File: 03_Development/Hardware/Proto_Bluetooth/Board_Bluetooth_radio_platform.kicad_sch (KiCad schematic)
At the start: 51 parts, among them J1 Conn_01x02, J10 Conn_01x03, J11 HMI_rotaryEncoder_1, J12 HMI_rotaryEncoder_1, J13 Conn_01x08_epaper, J17 Conn_01x02, J19 Conn_01x02_rn52_usb, J2 Conn_01x08, J3 BT_RN52_connector_left, J4 Conn_01x02, J5 BT_RN52_connector_right, J6 FM_interface, J7 BT_debug_connector, J8 BT_extension_connector, J9 SYS_debug_connector, SW1 SW_Push, U1 LM317_TO-220, U2 NXE2S1205MC

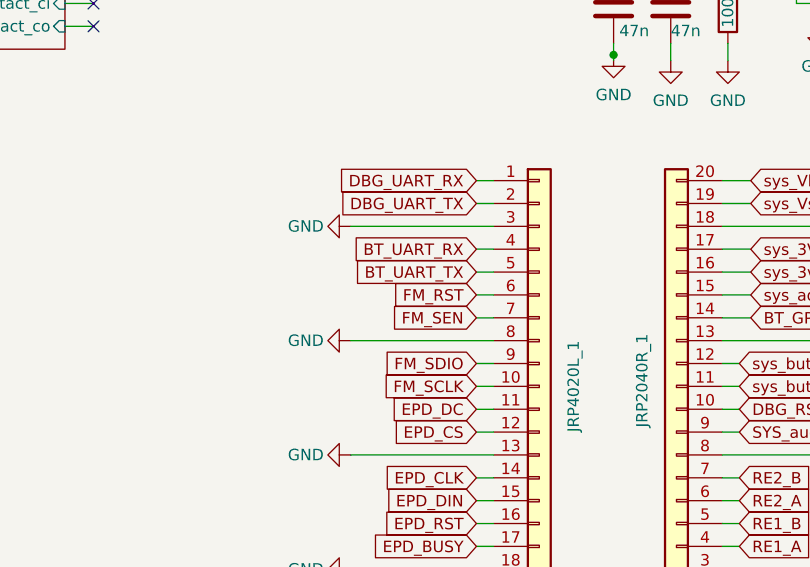
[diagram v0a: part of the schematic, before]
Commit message: [HDW_38] Fix Bt communication wires
Bluetooth Rx pin connected to GPIO4 of RP240
Bluetooth Tx pin connected to GPIO5 of RP2040
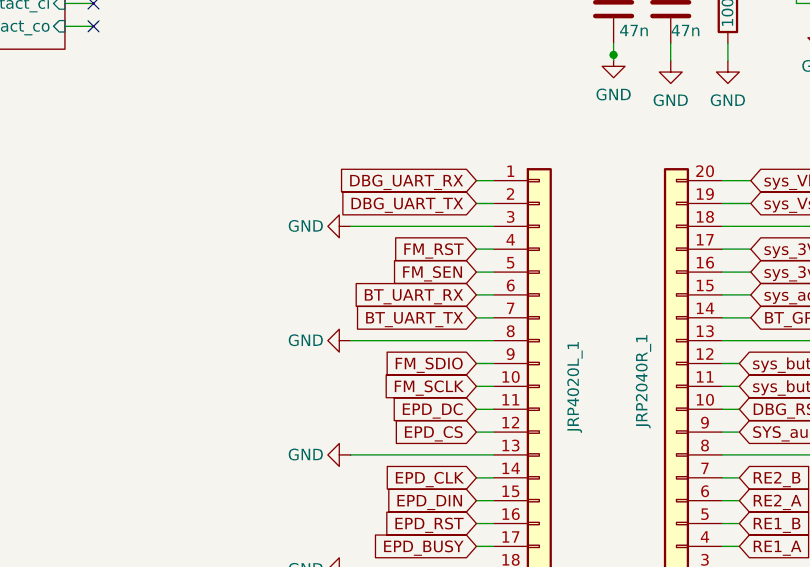
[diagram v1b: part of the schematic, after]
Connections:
- net BT_UART_RX: now also JRP4020L_1.6 (Pin_6); no longer JRP4020L_1.4 (Pin_4)
- net BT_UART_TX: now also JRP4020L_1.7 (Pin_7); no longer JRP4020L_1.5 (Pin_5)
- net FM_RST: now also JRP4020L_1.4 (Pin_4); no longer JRP4020L_1.6 (Pin_6)
- net FM_SEN: now also JRP4020L_1.5 (Pin_5); no longer JRP4020L_1.7 (Pin_7)
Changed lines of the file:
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@@
+    )
+  )
+  (global_label "BT_UART_RX" (shape input) (at 223.52 113.03 180) (fields_autoplaced)
+    (effects (font (size 1.27 1.27)) (justify right))
+    (property "Intersheet References" "${INTERSHEET_REFS}" (id 0) (at 209.7979 112.9506 0)
+      (effects (font (size 1.27 1.27)) (justify right) hide)
     )
   )
@@
     )
   )
-  (global_label "BT_UART_RX" (shape input) (at 223.52 107.95 180) (fields_autoplaced)
-    (effects (font (size 1.27 1.27)) (justify right))
-    (property "Intersheet References" "${INTERSHEET_REFS}" (id 0) (at 209.7979 107.8706 0)
+  (global_label "FM_SEN" (shape input) (at 223.52 110.49 180) (fields_autoplaced)
+    (effects (font (size 1.27 1.27)) (justify right))
+    (property "Intersheet References" "${INTERSHEET_REFS}" (id 0) (at 213.9102 110.4106 0)
+      (effects (font (size 1.27 1.27)) (justify right) hide)
+    )
+  )
+  (global_label "FM_RST" (shape input) (at 223.52 107.95 180) (fields_autoplaced)
+    (effects (font (size 1.27 1.27)) (justify right))
+    (property "Intersheet References" "${INTERSHEET_REFS}" (id 0) (at 214.1521 107.8706 0)
       (effects (font (size 1.27 1.27)) (justify right) hide)
     )
@@
     )
   )
-  (global_label "FM_RST" (shape input) (at 223.52 113.03 180) (fields_autoplaced)
-    (effects (font (size 1.27 1.27)) (justify right))
-    (property "Intersheet References" "${INTERSHEET_REFS}" (id 0) (at 214.1521 112.9506 0)
-      (effects (font (size 1.27 1.27)) (justify right) hide)
-    )
-  )
   (global_label "BT_PWREN" (shape input) (at 40.005 188.595 180) (fields_autoplaced)
     (effects (font (size 1.27 1.27)) (justify right))
@@
     )
   )
-  (global_label "FM_SEN" (shape input) (at 223.52 115.57 180) (fields_autoplaced)
-    (effects (font (size 1.27 1.27)) (justify right))
-    (property "Intersheet References" "${INTERSHEET_REFS}" (id 0) (at 213.9102 115.4906 0)
-      (effects (font (size 1.27 1.27)) (justify right) hide)
-    )
-  )
   (global_label "BT_MIC_R+" (shape input) (at 59.69 158.115 0) (fields_autoplaced)
     (effects (font (size 1.27 1.27)) (justify left))
@@
     )
   )
+  (global_label "BT_UART_TX" (shape input) (at 223.52 115.57 180) (fields_autoplaced)
+    (effects (font (size 1.27 1.27)) (justify right))
+    (property "Intersheet References" "${INTERSHEET_REFS}" (id 0) (at 210.1002 115.4906 0)
+      (effects (font (size 1.27 1.27)) (justify right) hide)
+    )
+  )
   (global_label "BT_SPI_SCK" (shape input) (at 59.69 173.355 0) (fields_autoplaced)
     (effects (font (size 1.27 1.27)) (justify left))
@@
       (effects (font (size 1.27 1.27)) (justify right) hide)
     )
-  )
-  (global_label "BT_UART_TX" (shape input) (at 223.52 110.49 180) (fields_autoplaced)
-    (effects (font (size 1.27 1.27)) (justify right))
-    (property "Intersheet References" "${INTERSHEET_REFS}" (id 0) (at 210.1002 110.4106 0)
-      (effects (font (size 1.27 1.27)) (justify right) hide)
-    )
